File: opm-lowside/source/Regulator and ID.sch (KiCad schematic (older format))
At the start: 11 parts, among them U401 LP2985-3.3, U402 AT25128B-SSHL-T8S1-L

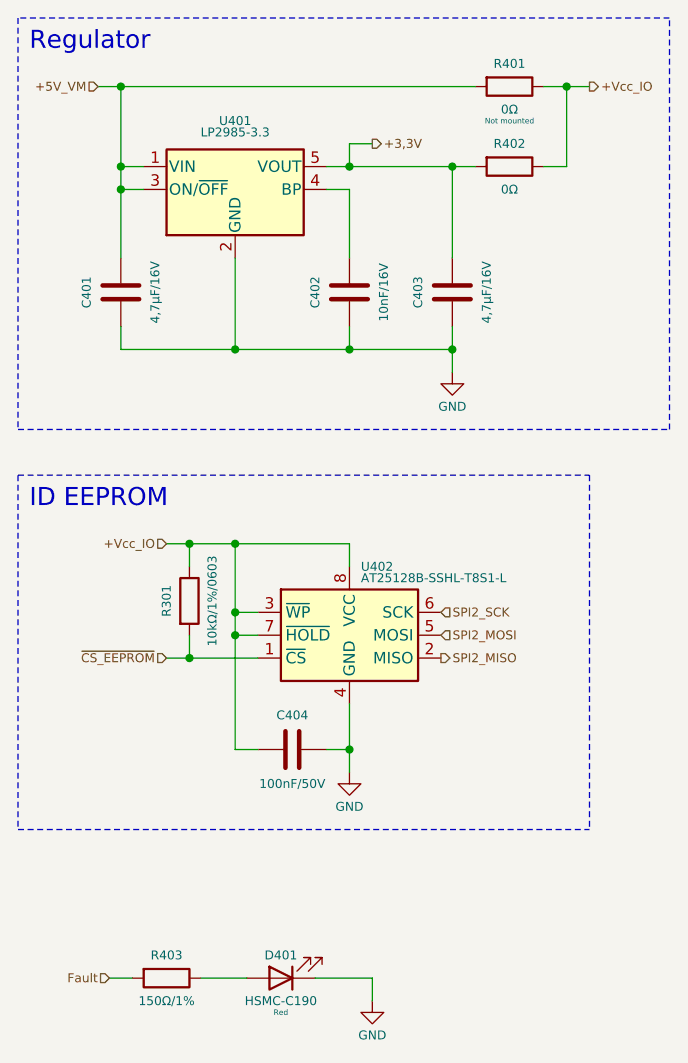
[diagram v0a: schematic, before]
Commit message: cleanup
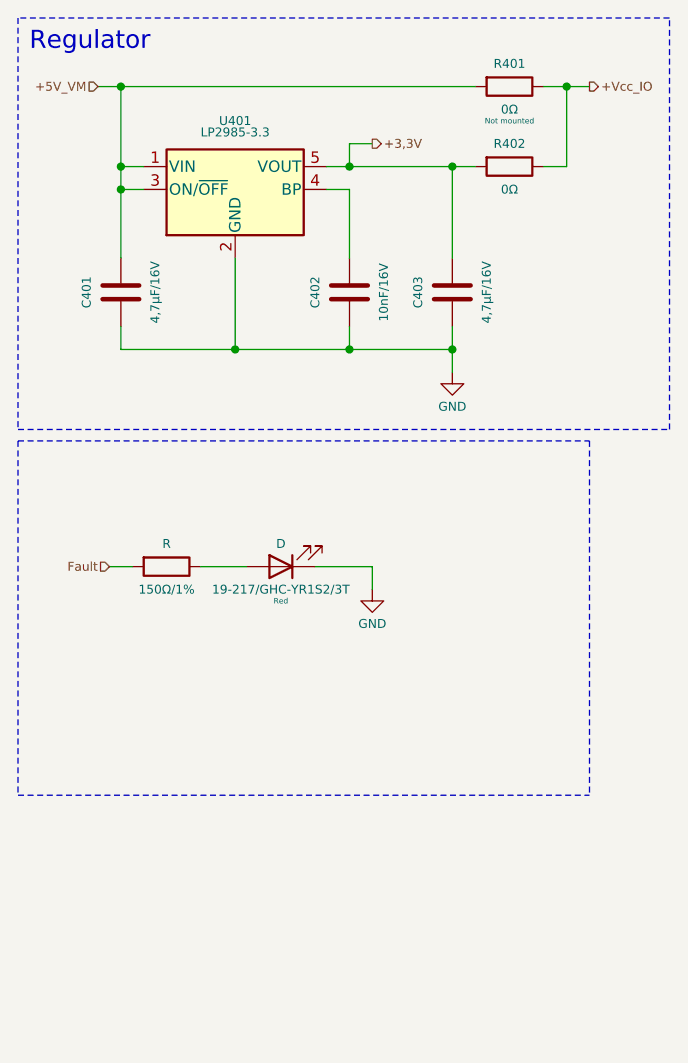
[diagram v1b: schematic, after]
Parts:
- removed C404: 100nF/50V, Capacitor_SMD:C_0603_1608Metric, symbol Device:C
- removed R301: 10kΩ/1%/0603, Resistor_SMD:R_0603_1608Metric, symbol Device:R
- removed U402: AT25128B-SSHL-T8S1-L, Package_SO:SOIC-8_3.9x4.9mm_P1.27mm, symbol opm-cache:Memory_EEPROM_AT25xxx
- D: renamed from D401; value HSMC-C190 -> 19-217/GHC-YR1S2/3T; LCSC (none) -> C72043; manf_num (none) -> 19-217/GHC-YR1S2/3T
- renumbered R403 to R
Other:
- note removed: "ID EEPROM"
- moved on the sheet: D, R
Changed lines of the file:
@@
 Comment4 ""
 $EndDescr
-Wire Wire Line
-	1950 2900 1950 2800
-Wire Wire Line
-	1450 2800 1450 3100
-Wire Wire Line
-	1450 3200 1550 3200
-Wire Wire Line
-	1550 3100 1450 3100
-Connection ~ 1450 3100
-Wire Wire Line
-	1450 3100 1450 3200
-Wire Wire Line
-	1450 2800 1250 2800
-$Comp
-L Device:C C?
-U 1 1 5D6ABCE6
-P 1700 3700
-AR Path="/5BA8C4E4/5D6ABCE6" Ref="C?"  Part="1"
-AR Path="/5D6A7BED/5D6ABCE6" Ref="C404"  Part="1"
-F 0 "C404" V 1550 3700 39  0000 C CNN
-F 1 "100nF/50V" V 1850 3700 39  0000 C CNN
-F 2 "Capacitor_SMD:C_0603_1608Metric" H 1738 3550 39  0001 C CNN
-F 3 "~" H 1700 3700 39  0001 C CNN
-	1    1700 3700
-	0    1    1    0
-$EndComp
-Connection ~ 1450 3200
-Wire Wire Line
-	1850 3700 1950 3700
-Wire Wire Line
-	1550 3700 1450 3700
-Wire Wire Line
-	1450 3200 1450 3700
-Wire Wire Line
-	1550 3300 1250 3300
-Text Notes 550  2650 0    79   ~ 0
-ID EEPROM
 $Comp
 L Regulator_Linear:LP2985-3.3 U401
@@
 	3350 500  500  500
 $Comp
-L Device:R R403
+L Device:R R
 U 1 1 5D67213B
-P 1150 4700
-F 0 "R403" V 1050 4700 39  0000 C CNN
-F 1 "150Ω/1%" V 1250 4700 39  0000 C CNN
-F 2 "Resistor_SMD:R_0603_1608Metric" V 1080 4700 39  0001 C CNN
-F 3 "~" H 1150 4700 39  0001 C CNN
-	1    1150 4700
+P 1150 2900
+F 0 "R" V 1050 2900 39  0000 C CNN
+F 1 "150Ω/1%" V 1250 2900 39  0000 C CNN
+F 2 "Resistor_SMD:R_0603_1608Metric" V 1080 2900 39  0001 C CNN
+F 3 "~" H 1150 2900 39  0001 C CNN
+F 4 "" V 1150 2900 50  0001 C CNN "Field4"
+F 5 "" V 1150 2900 50  0001 C CNN "Field5"
+	1    1150 2900
 	0    1    1    0
 $EndComp
 $Comp
-L Device:LED D401
+L Device:LED D
 U 1 1 5D67284F
-P 1650 4700
-F 0 "D401" H 1650 4600 39  0000 C CNN
-F 1 "HSMC-C190" H 1650 4800 39  0000 C CNN
-F 2 "LED_SMD:LED_0603_1608Metric" H 1650 4700 39  0001 C CNN
-F 3 "~" H 1650 4700 39  0001 C CNN
-F 4 "Red" H 1650 4850 24  0000 C CNN "Info"
-	1    1650 4700
+P 1650 2900
+F 0 "D" H 1650 2800 39  0000 C CNN
+F 1 "19-217/GHC-YR1S2/3T" H 1650 3000 39  0000 C CNN
+F 2 "LED_SMD:LED_0603_1608Metric" H 1650 2900 39  0001 C CNN
+F 3 "https://datasheet.lcsc.com/lcsc/1811101510_Everlight-Elec-19-217-GHC-YR1S2-3T_C72043.pdf" H 1650 2900 39  0001 C CNN
+F 4 "Red" H 1650 3050 24  0000 C CNN "Info"
+F 5 "C72043" H 1650 2900 50  0001 C CNN "LCSC"
+F 6 "19-217/GHC-YR1S2/3T" H 1650 2900 50  0001 C CNN "manf_num"
+	1    1650 2900
 	-1   0    0    1
 $EndComp
-Text HLabel 900  4700 0    39   Input ~ 0
+Text HLabel 900  2900 0    39   Input ~ 0
 Fault
 Wire Wire Line
-	1300 4700 1500 4700
-Wire Wire Line
-	1800 4700 2050 4700
-Wire Wire Line
-	2050 4700 2050 4800
+	1300 2900 1500 2900
+Wire Wire Line
+	1800 2900 2050 2900
+Wire Wire Line
+	2050 2900 2050 3000
 $Comp
 L power:GND #PWR0130
 U 1 1 5D67425C
-P 2050 4800
-F 0 "#PWR0130" H 2050 4550 39  0001 C CNN
-F 1 "GND" H 2050 4650 39  0000 C CNN
-F 2 "" H 2050 4800 39  0001 C CNN
-F 3 "" H 2050 4800 39  0001 C CNN
-	1    2050 4800
-	1    0    0    -1
-$EndComp
-Wire Wire Line
-	900  4700 1000 4700
-Text HLabel 1150 3300 0    39   Input ~ 0
-~CS_EEPROM
-Text HLabel 2350 3100 2    39   Input ~ 0
-SPI2_SCK
-Connection ~ 1450 2800
-Wire Wire Line
-	1950 3700 1950 3500
-Wire Wire Line
-	1950 2800 1450 2800
-$Comp
-L opm-cache:Memory_EEPROM_AT25xxx U402
-U 1 1 5D6ABCD6
-P 1950 3200
-F 0 "U402" H 2000 3500 39  0000 L CNN
-F 1 "AT25128B-SSHL-T8S1-L" H 2000 3450 39  0000 L CNN
-F 2 "Package_SO:SOIC-8_3.9x4.9mm_P1.27mm" H 1950 3200 39  0001 C CNN
-F 3 "http://ww1.microchip.com/downloads/en/DeviceDoc/Atmel-8707-SEEPROM-AT25010B-020B-040B-Datasheet.pdf" H 1950 3200 39  0001 C CNN
-	1    1950 3200
-	1    0    0    -1
-$EndComp
-Text HLabel 2350 3200 2    39   Input ~ 0
-SPI2_MOSI
-Text HLabel 2350 3300 2    39   Output ~ 0
-SPI2_MISO
-Text HLabel 1150 2800 0    39   Input ~ 0
-+Vcc_IO
+P 2050 3000
+F 0 "#PWR0130" H 2050 2750 39  0001 C CNN
+F 1 "GND" H 2050 2850 39  0000 C CNN
+F 2 "" H 2050 3000 39  0001 C CNN
+F 3 "" H 2050 3000 39  0001 C CNN
+	1    2050 3000
+	1    0    0    -1
+$EndComp
+Wire Wire Line
+	900  2900 1000 2900
 Text HLabel 2050 1050 2    39   Output ~ 0
 +3,3V
@@
 Wire Wire Line
 	1950 1150 2400 1150
-$Comp
-L power:GND #PWR0301
-U 1 1 5DCD3733
-P 1950 3800
-F 0 "#PWR0301" H 1950 3550 39  0001 C CNN
-F 1 "GND" H 1950 3650 39  0000 C CNN
-F 2 "" H 1950 3800 39  0001 C CNN
-F 3 "" H 1950 3800 39  0001 C CNN
-	1    1950 3800
-	1    0    0    -1
-$EndComp
-Wire Wire Line
-	1950 3800 1950 3700
-Connection ~ 1950 3700
-Wire Notes Line
-	500  2500 3000 2500
-Wire Notes Line
-	500  4050 3000 4050
-Wire Notes Line
-	3000 2500 3000 4050
-Wire Notes Line
-	500  2500 500  4050
-$Comp
-L Device:R R301
-U 1 1 5DF96ED6
-P 1250 3050
-F 0 "R301" V 1150 3050 39  0000 C CNN
-F 1 "10kΩ/1%/0603" V 1350 3050 39  0000 C CNN
-F 2 "Resistor_SMD:R_0603_1608Metric" V 1180 3050 39  0001 C CNN
-F 3 "~" H 1250 3050 39  0001 C CNN
-	1    1250 3050
-	1    0    0    -1
-$EndComp
-Wire Wire Line
-	1250 2900 1250 2800
-Connection ~ 1250 2800
-Wire Wire Line
-	1250 2800 1150 2800
-Wire Wire Line
-	1250 3200 1250 3300
-Connection ~ 1250 3300
-Wire Wire Line
-	1250 3300 1150 3300
+Wire Notes Line
+	500  2350 3000 2350
+Wire Notes Line
+	3000 2350 3000 3900
+Wire Notes Line
+	500  3900 3000 3900
+Wire Notes Line
+	500  2350 500  3900
 $EndSCHEMATC
